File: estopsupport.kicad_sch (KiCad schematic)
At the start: 27 parts, among them J1 Barrier Block 1x3, J2 Dupont 1x2, J3 Dupont 1x2, J4 Dupont 1x2, J5 Dupont 2x4, K1 QLRELAY JQX-V7H 012-1HP, Q1 2N7002, U1 BTS6163D, U2 PC817

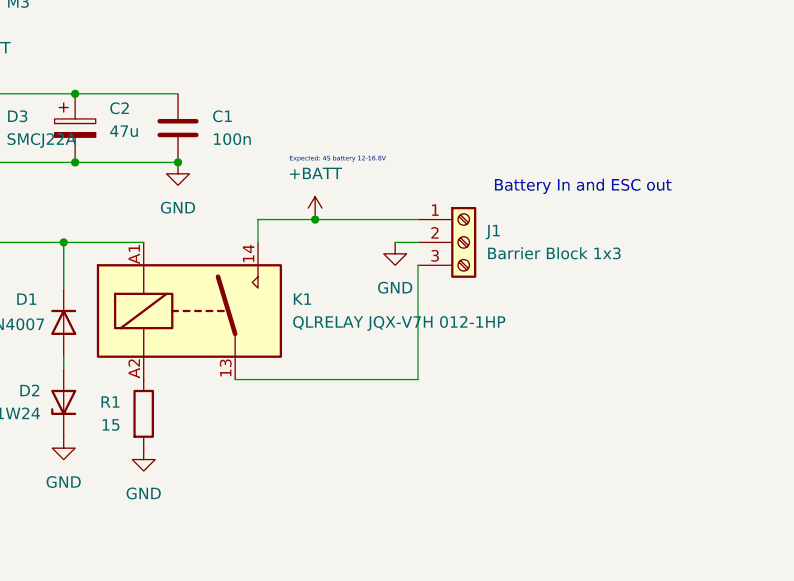
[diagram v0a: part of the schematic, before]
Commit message: layout rework
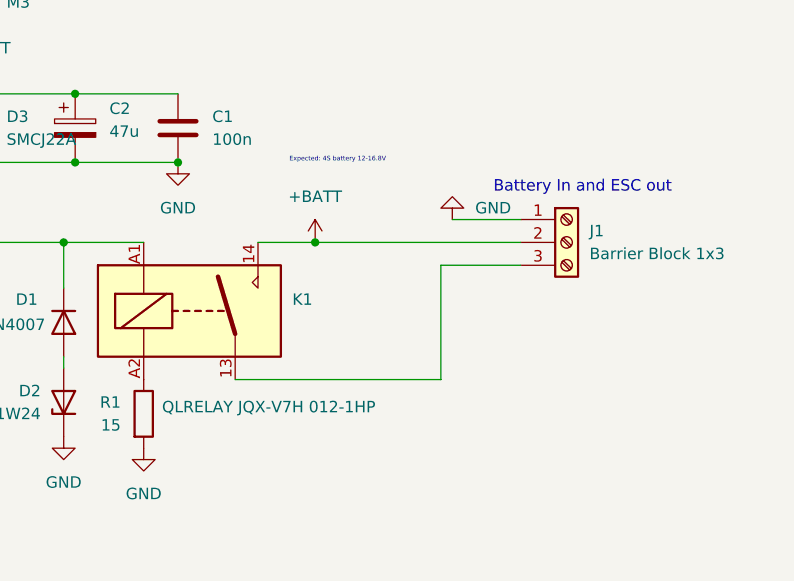
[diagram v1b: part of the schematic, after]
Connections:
- net +BATT: now also J1.2 (Pin_2); no longer J1.1 (Pin_1)
- net GND: now also J1.1 (Pin_1); no longer J1.2 (Pin_2)
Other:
- moved on the sheet: J1
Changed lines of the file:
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@@
 	)
 	(junction
-		(at 138.43 63.5)
-		(diameter 0)
-		(color 0 0 0 0)
-	)
-	(junction
 		(at 34.29 96.52)
 		(diameter 0)
@@
 	)
 	(junction
+		(at 138.43 66.04)
+		(diameter 0)
+		(color 0 0 0 0)
+	)
+	(junction
 		(at 111.76 49.53)
 		(diameter 0)
@@
 	(wire
 		(pts
+			(xy 138.43 66.04) (xy 161.29 66.04)
+		)
+		(stroke
+			(width 0)
+			(type default)
+		)
+	)
+	(wire
+		(pts
 			(xy 48.26 63.5) (xy 50.8 63.5)
 		)
@@
 	(wire
 		(pts
-			(xy 110.49 78.74) (xy 110.49 80.01)
+			(xy 153.67 63.5) (xy 161.29 63.5)
 		)
 		(stroke
@@
 	(wire
 		(pts
-			(xy 21.59 63.5) (xy 26.67 63.5)
+			(xy 110.49 78.74) (xy 110.49 80.01)
 		)
 		(stroke
@@
 	(wire
 		(pts
-			(xy 132.08 66.04) (xy 132.08 63.5)
+			(xy 21.59 63.5) (xy 26.67 63.5)
 		)
 		(stroke
@@
 	(wire
 		(pts
-			(xy 34.29 93.98) (xy 34.29 96.52)
+			(xy 152.4 68.58) (xy 161.29 68.58)
 		)
 		(stroke
@@
 	(wire
 		(pts
-			(xy 21.59 53.34) (xy 21.59 60.96)
+			(xy 34.29 93.98) (xy 34.29 96.52)
 		)
 		(stroke
@@
 	(wire
 		(pts
-			(xy 129.54 81.28) (xy 149.86 81.28)
+			(xy 21.59 53.34) (xy 21.59 60.96)
 		)
 		(stroke
@@
 	(wire
 		(pts
-			(xy 149.86 68.58) (xy 149.86 81.28)
+			(xy 129.54 81.28) (xy 152.4 81.28)
 		)
 		(stroke
@@
 	(wire
 		(pts
-			(xy 101.6 49.53) (xy 111.76 49.53)
+			(xy 152.4 68.58) (xy 152.4 81.28)
 		)
 		(stroke
@@
 	(wire
 		(pts
-			(xy 26.67 96.52) (xy 34.29 96.52)
+			(xy 101.6 49.53) (xy 111.76 49.53)
 		)
 		(stroke
@@
 	(wire
 		(pts
-			(xy 93.98 48.26) (xy 93.98 49.53)
+			(xy 26.67 96.52) (xy 34.29 96.52)
 		)
 		(stroke
@@
 	(wire
 		(pts
-			(xy 34.29 83.82) (xy 45.72 83.82)
+			(xy 93.98 48.26) (xy 93.98 49.53)
 		)
 		(stroke
@@
 	(wire
 		(pts
-			(xy 82.55 69.85) (xy 82.55 68.58)
+			(xy 34.29 83.82) (xy 45.72 83.82)
 		)
 		(stroke
@@
 	(wire
 		(pts
-			(xy 147.32 66.04) (xy 149.86 66.04)
+			(xy 82.55 69.85) (xy 82.55 68.58)
 		)
 		(stroke
@@
 	(wire
 		(pts
-			(xy 138.43 63.5) (xy 149.86 63.5)
-		)
-		(stroke
-			(width 0)
-			(type default)
-		)
-	)
-	(wire
-		(pts
 			(xy 110.49 66.04) (xy 110.49 71.12)
 		)
@@
 	(wire
 		(pts
-			(xy 132.08 63.5) (xy 138.43 63.5)
+			(xy 132.08 66.04) (xy 138.43 66.04)
 		)
 		(stroke
@@
 		(length 2.54)
 		(shape round)
-		(at 149.86 81.28 180)
+		(at 152.4 81.28 180)
 		(fields_autoplaced yes)
 		(effects
@@
 		)
 		(property "Netclass" "Power"
-			(at 150.5585 83.82 0)
+			(at 153.0985 83.82 0)
 			(show_name no)
 			(do_not_autoplace no)
@@
 		)
 		(property "Component Class" ""
-			(at -46.99 25.4 0)
+			(at -44.45 25.4 0)
 			(show_name no)
 			(do_not_autoplace no)
@@
 	(symbol
 		(lib_id "power:GND")
-		(at 147.32 66.04 0)
+		(at 153.67 63.5 180)
 		(unit 1)
 		(body_style 1)
@@
 		(fields_autoplaced yes)
 		(property "Reference" "#PWR07"
-			(at 147.32 72.39 0)
+			(at 153.67 57.15 0)
 			(hide yes)
 			(show_name no)
@@
 		)
 		(property "Value" "GND"
-			(at 147.32 71.12 0)
+			(at 156.21 62.2299 0)
 			(show_name no)
 			(do_not_autoplace no)
@@
 					(size 1.27 1.27)
 				)
+				(justify right)
 			)
 		)
 		(property "Footprint" ""
-			(at 147.32 66.04 0)
+			(at 153.67 63.5 0)
 			(hide yes)
 			(show_name no)
@@
 		)
 		(property "Datasheet" ""
-			(at 147.32 66.04 0)
+			(at 153.67 63.5 0)
 			(hide yes)
 			(show_name no)
@@
 		)
 		(property "Description" "Power symbol creates a global label with name \"GND\" , ground"
-			(at 147.32 66.04 0)
+			(at 153.67 63.5 0)
 			(hide yes)
 			(show_name no)
@@
 	(symbol
 		(lib_id "Connector:Screw_Terminal_01x03")
-		(at 154.94 66.04 0)
+		(at 166.37 66.04 0)
 		(unit 1)
 		(body_style 1)
@@
 		(fields_autoplaced yes)
 		(property "Reference" "J1"
-			(at 157.48 64.7699 0)
+			(at 168.91 64.7699 0)
 			(show_name no)
 			(do_not_autoplace no)
@@
 		)
 		(property "Value" "Barrier Block 1x3"
-			(at 157.48 67.3099 0)
+			(at 168.91 67.3099 0)
 			(show_name no)
 			(do_not_autoplace no)
@@
 		)
 		(property "Footprint" "EasyEDA_Lib:CONN-TH_KF88SA-16.0-3P"
-			(at 154.94 66.04 0)
+			(at 166.37 66.04 0)
 			(hide yes)
 			(show_name no)
@@
 		)
 		(property "Datasheet" ""
-			(at 154.94 66.04 0)
+			(at 166.37 66.04 0)
 			(hide yes)
 			(show_name no)
@@
 		)
 		(property "Description" "Generic screw terminal, single row, 01x03, script generated (kicad-library-utils/schlib/autogen/connector/)"
-			(at 154.94 66.04 0)
+			(at 166.37 66.04 0)
 			(hide yes)
 			(show_name no)
@@
 		)
 		(property "Sim.Device" "V"
-			(at 154.94 66.04 0)
+			(at 166.37 66.04 0)
 			(hide yes)
 			(show_name no)
@@
 		)
 		(property "Sim.Type" "DC"
-			(at 154.94 66.04 0)
+			(at 166.37 66.04 0)
 			(hide yes)
 			(show_name no)
@@
 		)
 		(property "Sim.Pins" "1=+ 2=-"
-			(at 154.94 66.04 0)
+			(at 166.37 66.04 0)
 			(hide yes)
 			(show_name no)
@@
 		)
 		(property "Sim.Params" "dc=12"
-			(at 154.94 66.04 0)
+			(at 166.37 66.04 0)
 			(hide yes)
 			(show_name no)
@@
 		)
 		(property "JLCPCB Part #" ""
-			(at 154.94 66.04 0)
+			(at 166.37 66.04 0)
 			(hide yes)
 			(show_name no)
@@
 		(in_pos_files yes)
 		(dnp no)
-		(fields_autoplaced yes)
 		(property "Reference" "K1"
 			(at 135.89 72.3899 0)
@@
 		)
 		(property "Value" "QLRELAY JQX-V7H 012-1HP"
-			(at 135.89 74.9299 0)
+			(at 121.412 84.328 0)
 			(show_name no)
 			(do_not_autoplace no)
@@
 	(symbol
 		(lib_id "power:+BATT")
-		(at 138.43 63.5 0)
+		(at 138.43 66.04 0)
 		(unit 1)
 		(body_style 1)
@@
 		(fields_autoplaced yes)
 		(property "Reference" "#PWR02"
-			(at 138.43 67.31 0)
+			(at 138.43 69.85 0)
 			(hide yes)
 			(show_name no)
@@
 		)
 		(property "Value" "+BATT"
-			(at 138.43 58.42 0)
+			(at 138.43 60.96 0)
 			(show_name no)
 			(do_not_autoplace no)
@@
 		)
 		(property "Footprint" ""
-			(at 138.43 63.5 0)
+			(at 138.43 66.04 0)
 			(hide yes)
 			(show_name no)
@@
 		)
 		(property "Datasheet" ""
-			(at 138.43 63.5 0)
+			(at 138.43 66.04 0)
 			(hide yes)
 			(show_name no)
@@
 		)
 		(property "Description" "Power symbol creates a global label with name \"+BATT\""
-			(at 138.43 63.5 0)
+			(at 138.43 66.04 0)
 			(hide yes)
 			(show_name no)
